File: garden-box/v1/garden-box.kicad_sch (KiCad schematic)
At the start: 17 parts, among them J1 USB_A, J2 Conn_01x03_Male, J3 Conn_01x04_Male, J4 Screw_Terminal_01x02, J5 Screw_Terminal_01x02, J6 Screw_Terminal_01x02, K1 G6DN-1A-L_DC5, Q1 2N3904, T1 Transformer_1P_2S, U1 ESP32-POE

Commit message: update footprint on PCB
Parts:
- T1: footprint rs-online:VCM36212 -> mylife-footprints:VCM36212
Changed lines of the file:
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@@
     (property "Reference" "T1" (id 0) (at 246.38 85.0603 0))
     (property "Value" "Transformer_1P_2S" (id 1) (at 246.38 87.8354 0))
-    (property "Footprint" "rs-online:VCM36212" (id 2) (at 246.38 99.06 0)
+    (property "Footprint" "mylife-footprints:VCM36212" (id 2) (at 246.38 99.06 0)
       (effects (font (size 1.27 1.27)) hide)
     )
@@
     )
     (path "/be49853a-e63a-418f-add4-0398acbca9cd"
-      (reference "T1") (unit 1) (value "Transformer_1P_2S") (footprint "rs-online:VCM36212")
+      (reference "T1") (unit 1) (value "Transformer_1P_2S") (footprint "mylife-footprints:VCM36212")
     )
     (path "/a51d3ce6-8227-462c-b55f-ac7604ee63f5"

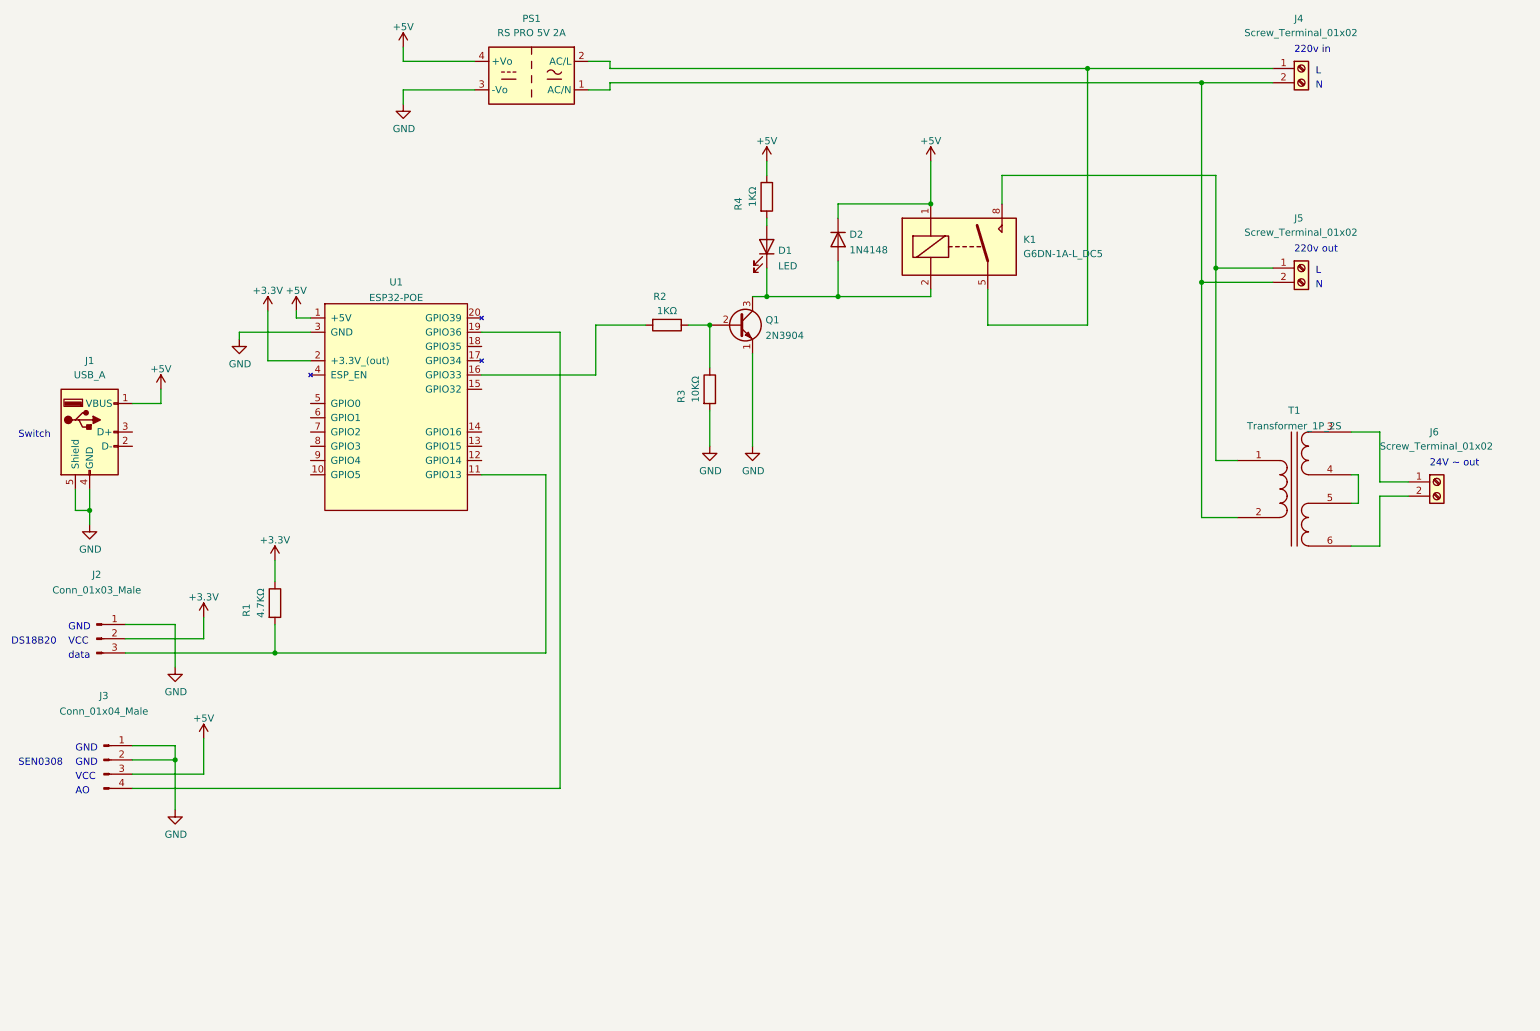
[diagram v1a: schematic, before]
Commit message: wip v1 layout
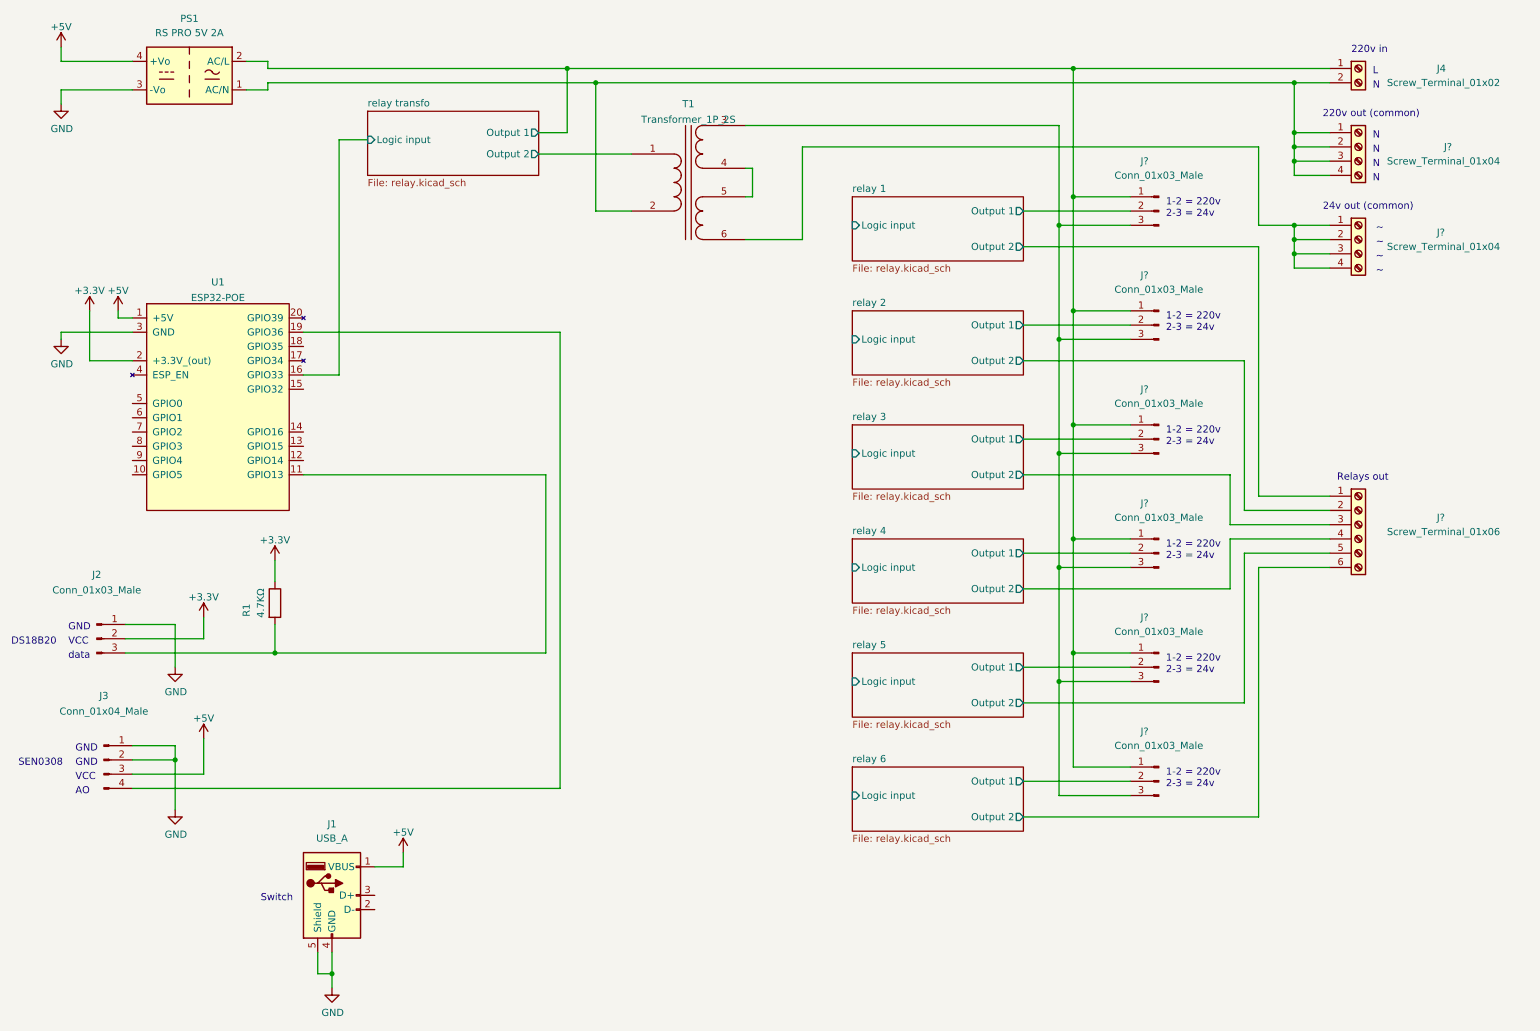
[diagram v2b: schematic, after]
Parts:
- removed D1: LED, Diode_SMD:D_0805_2012Metric, symbol Device:LED
- removed D2: 1N4148, Diode_SMD:D_SOD-123, symbol Diode:1N4148
- removed J5, J6: Screw_Terminal_01x02, TerminalBlock:TerminalBlock_bornier-2_P5.08mm, symbol Connector:Screw_Terminal_01x02
- removed K1: G6DN-1A-L_DC5, rs-online:G6DN-1A-L, symbol mylife-symbols:G6DN-1A-L_DC5
- removed Q1: 2N3904, jlcpcb:SOT-23-3_L2.9-W1.3-P1.90-LS2.4-TR, symbol Transistor_BJT:2N3904
- removed R2, R4: 1KΩ, Resistor_SMD:R_0402_1005Metric, symbol Device:R
- removed R3: 10KΩ, Resistor_SMD:R_0402_1005Metric, symbol Device:R
- added J? (x6): Conn_01x03_Male, Connector_PinHeader_2.54mm:PinHeader_1x03_P2.54mm_Vertical, symbol Connector:Conn_01x03_Male
- added J?: Screw_Terminal_01x06, TerminalBlock:TerminalBlock_bornier-2_P5.08mm, symbol Connector:Screw_Terminal_01x06
- added J? (x2): Screw_Terminal_01x04, TerminalBlock:TerminalBlock_bornier-2_P5.08mm, symbol Connector:Screw_Terminal_01x04
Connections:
- net at J4.2 (Pin_2), PS1.1 (AC/N), T1.2 (AB): now also J?.1 (Pin_1), J?.2 (Pin_2), J?.3 (Pin_3), J?.4 (Pin_4)
- net relay transfo/Output 1: now reaches J4.1 (Pin_1), PS1.2 (AC/L)
- net relay transfo/Output 1: now also J?.1 (Pin_1), J?.1 (Pin_1), J?.1 (Pin_1), J?.1 (Pin_1), J?.1 (Pin_1), J?.1 (Pin_1)
- net relay transfo/Logic input: now reaches U1.16 (GPIO33)
- net relay transfo/Output 2: now reaches T1.1 (AA)
- net at T1.3 (SA): now also J?.3 (Pin_3), J?.3 (Pin_3), J?.3 (Pin_3), J?.3 (Pin_3), J?.3 (Pin_3), J?.3 (Pin_3)
- net at T1.6 (SD): now also J?.1 (Pin_1), J?.2 (Pin_2), J?.3 (Pin_3), J?.4 (Pin_4)
- new net relay 1/Output 1: J?.2 (Pin_2)
- new net relay 1/Output 2: J?.1 (Pin_1)
- new net relay 2/Output 1: J?.2 (Pin_2)
- new net relay 2/Output 2: J?.2 (Pin_2)
- new net relay 3/Output 1: J?.2 (Pin_2)
- new net relay 3/Output 2: J?.3 (Pin_3)
- new net relay 4/Output 1: J?.2 (Pin_2)
- new net relay 4/Output 2: J?.4 (Pin_4)
- new net relay 5/Output 1: J?.2 (Pin_2)
- new net relay 5/Output 2: J?.5 (Pin_5)
- new net relay 6/Output 1: J?.2 (Pin_2)
- new net relay 6/Output 2: J?.6 (Pin_6)
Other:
- added sheet relay 1 (relay.kicad_sch)
- added sheet relay 2 (relay.kicad_sch)
- added sheet relay 3 (relay.kicad_sch)
- added sheet relay 4 (relay.kicad_sch)
- added sheet relay 5 (relay.kicad_sch)
- added sheet relay 6 (relay.kicad_sch)
- added sheet relay transfo (relay.kicad_sch)
- note added: "1-2 = 220v 2-3 = 24v"
- note added: "220v out (common)"
- note added: "24v out (common)"
- note added: "Relays out"
- note added: "~"
- note removed: "220v out"
- note removed: "24V ~ out"
- moved on the sheet: J1, J4, PS1, T1, U1
